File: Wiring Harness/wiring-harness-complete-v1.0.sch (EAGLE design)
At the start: 36 parts, among them J1 M80-879, J10 SMA-142-0701-801/806, J11 SMA-142-0701-801/806, J12 SMA-142-0701-801/806, J13 SMA-142-0701-801/806, J16 SMA-142-0701-801/806, J17 SMA-142-0701-801/806, J18 SMA-142-0701-871/880, J19 SMA-142-0701-871/880, J2 M80-5000000M1-10-331-000, J20 GLENAIR-171-006-6-S-6-7-18, J21 GLENAIR-171-006-6-S-6-7-18, J22 GLENAIR-171-006-6-S-6-7-18, J23 GLENAIR-171-006-6-S-6-7-18, J3 M80-5000000M1-10-331-00-000, J30 M80-866XXXX, J31 M80-866XXXX, J4 SMFC, J50 22-27-2021-02, J53 22-05-7028-02, SW1 CT10-XXXX-A2, SW2 CT10-XXXX-A2, SW3 CT10-XXXX-A2, X16 5566-14

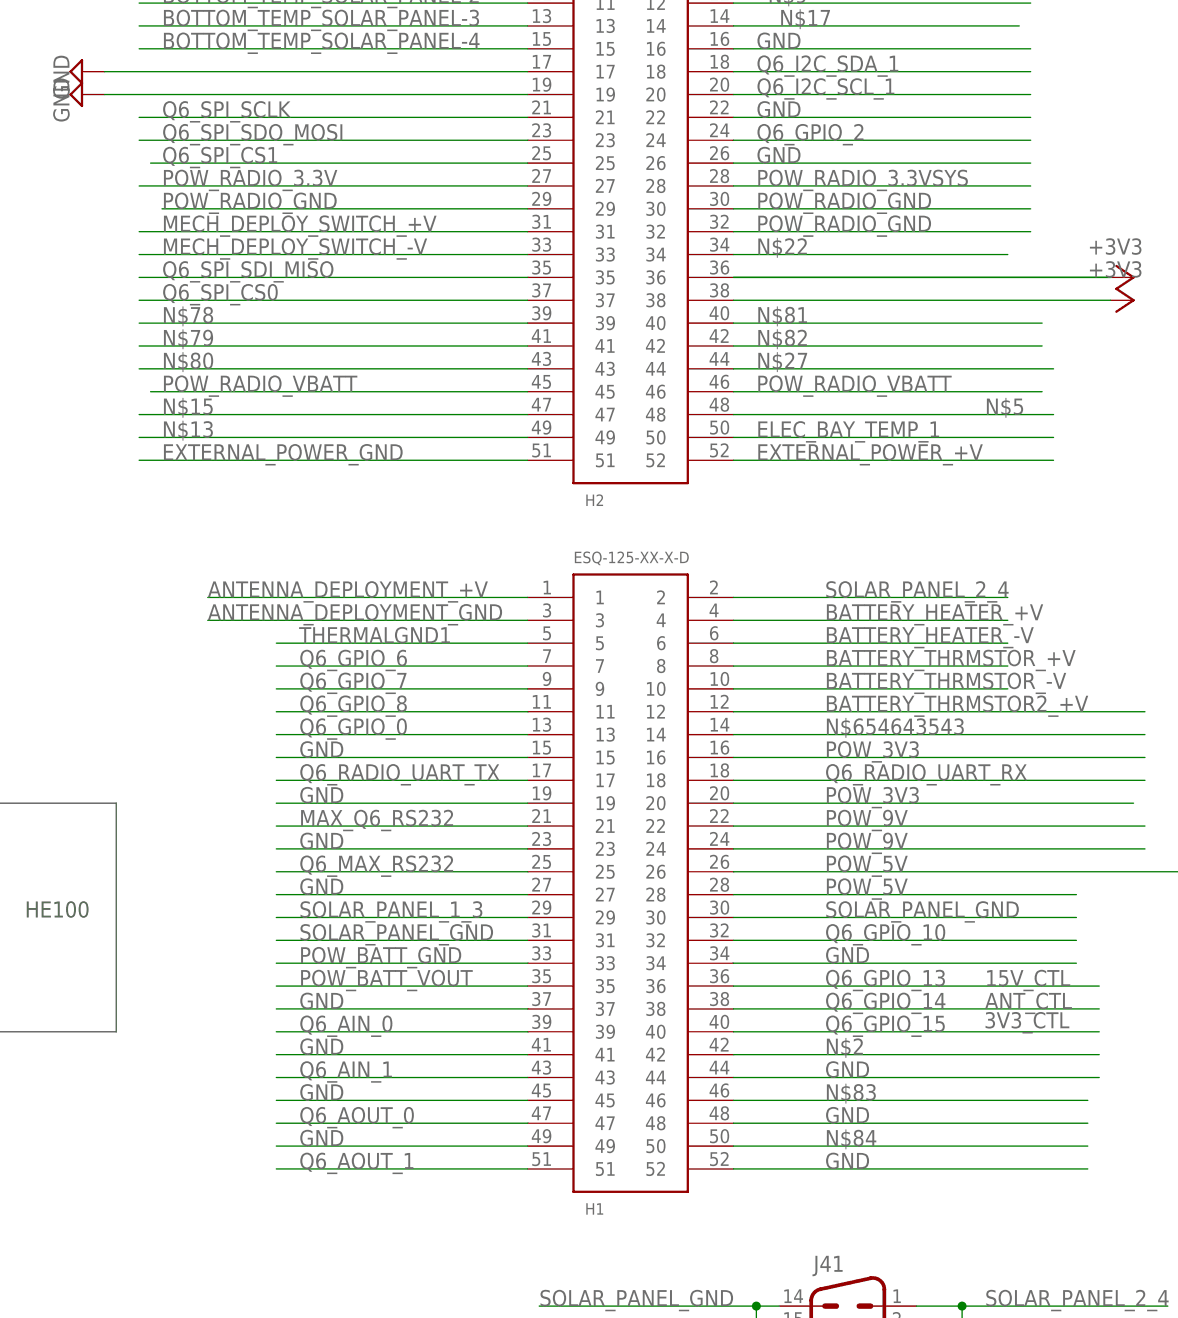
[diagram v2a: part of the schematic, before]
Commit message: [Wiring Harness] [Payload-Internal-Aux] Renamed unconnected header pins to match wiring harness. The remaining conflicts are legitimate wired net conflicts and can only be resolved with redesign.
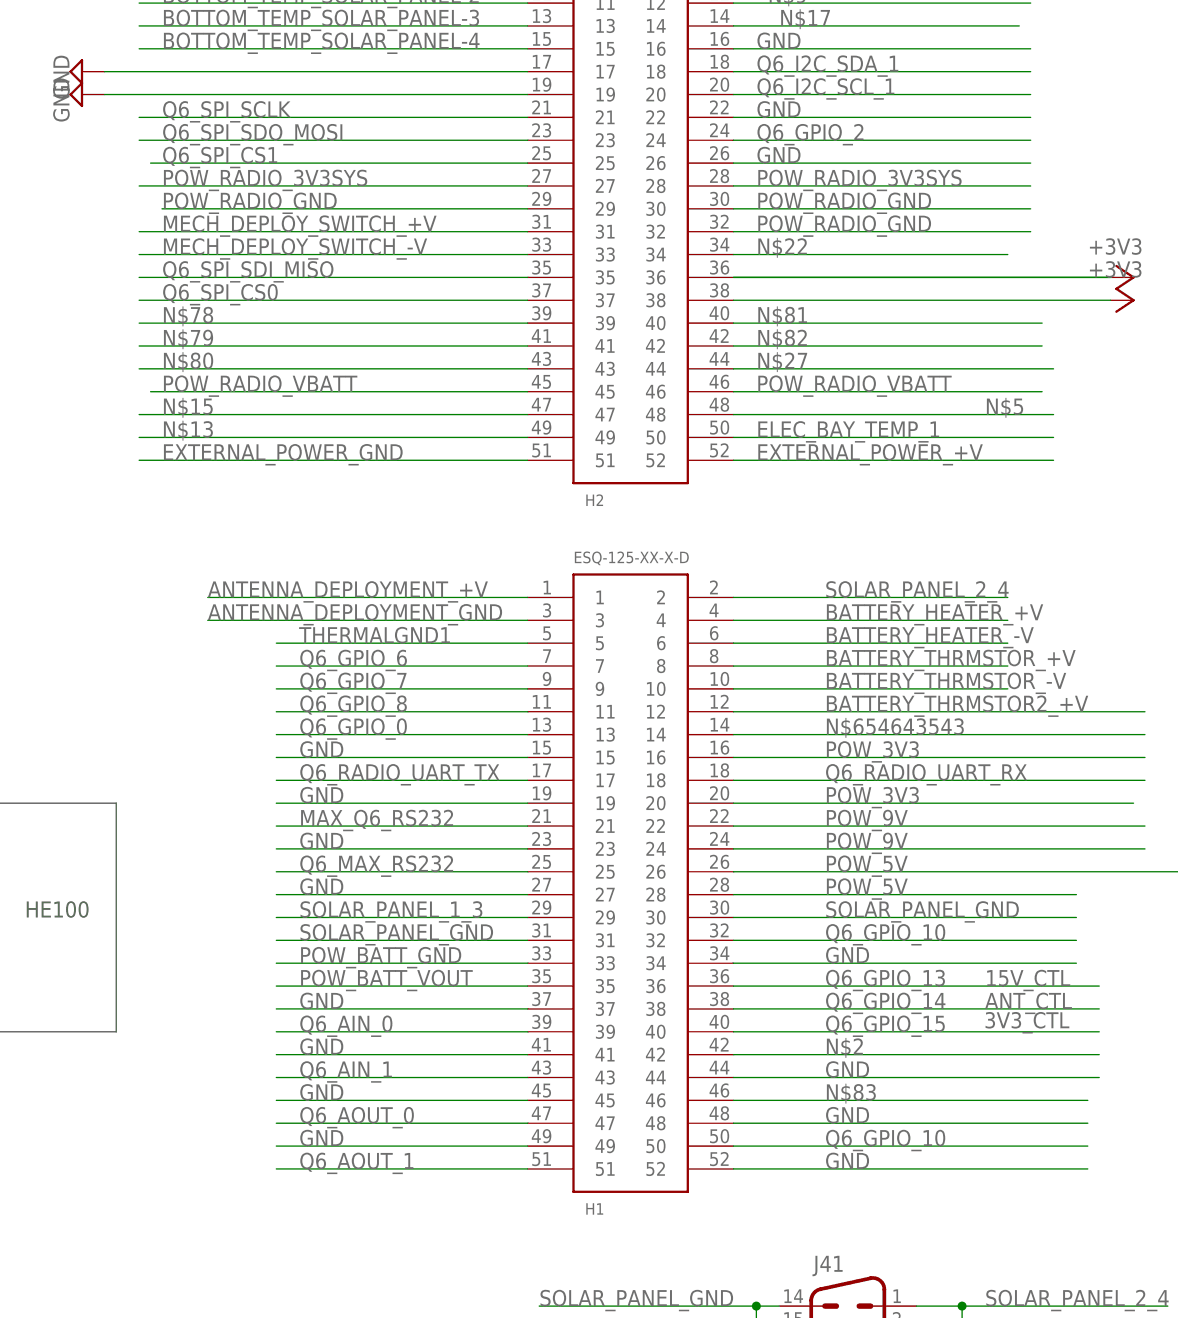
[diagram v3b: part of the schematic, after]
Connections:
- removed net N$84: H1.50
- removed net POW_RADIO_3.3V: H2.27
- removed net POW_RADIO_3.3VSYS: H2.28
- new net POW_RADIO_3V3SYS: H2.27, H2.28
- net Q6_GPIO_10: now also H1.50
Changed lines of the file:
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@@
 </segment>
 </net>
-<net name="POW_RADIO_3.3VSYS" class="0">
+<net name="POW_RADIO_3V3SYS" class="0">
 <segment>
 <pinref part="H2" gate="G$1" pin="28"/>
 <wire x1="7.62" y1="0" x2="40.64" y2="0" width="0.1524" layer="91"/>
 <label x="10.16" y="0" size="1.778" layer="95"/>
+</segment>
+<segment>
+<pinref part="H2" gate="G$1" pin="27"/>
+<wire x1="-15.24" y1="0" x2="-58.42" y2="0" width="0.1524" layer="91"/>
+<label x="-55.88" y="0" size="1.778" layer="95"/>
 </segment>
 </net>
@@
 </segment>
 </net>
-<net name="POW_RADIO_3.3V" class="0">
-<segment>
-<pinref part="H2" gate="G$1" pin="27"/>
-<wire x1="-15.24" y1="0" x2="-58.42" y2="0" width="0.1524" layer="91"/>
-<label x="-55.88" y="0" size="1.778" layer="95"/>
-</segment>
-</net>
 <net name="POW_3V3" class="0">
 <segment>
@@
 <wire x1="52.07" y1="109.22" x2="22.86" y2="109.22" width="0.1524" layer="91"/>
 <label x="35.56" y="109.22" size="1.778" layer="95"/>
+</segment>
+<segment>
+<pinref part="H1" gate="G$1" pin="50"/>
+<wire x1="7.62" y1="-106.68" x2="46.99" y2="-106.68" width="0.1524" layer="91"/>
+<label x="17.78" y="-106.68" size="1.778" layer="95"/>
 </segment>
 </net>
@@
 </segment>
 </net>
-<net name="N$84" class="0">
-<segment>
-<pinref part="H1" gate="G$1" pin="50"/>
-<wire x1="7.62" y1="-106.68" x2="46.99" y2="-106.68" width="0.1524" layer="91"/>
-<label x="17.78" y="-106.68" size="1.778" layer="95"/>
-</segment>
-</net>
